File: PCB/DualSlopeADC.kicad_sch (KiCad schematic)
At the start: 25 parts, among them J2 Conn_01x02_Pin, J3 Conn_01x02_Pin, J5 Conn_01x02_Pin, J6 Conn_01x02_Pin, J7 Conn_01x02_Pin, J8 Conn_01x02_Pin, J9 Conn_01x02_Pin, U1 CH32V003FxPx, U2 ADR4533, U3 AD8605ARTZ-R2, U4 ADG419BRM, U5 LTC6752xSC6-4, U6 CA56-12EWA, U7 AD8656

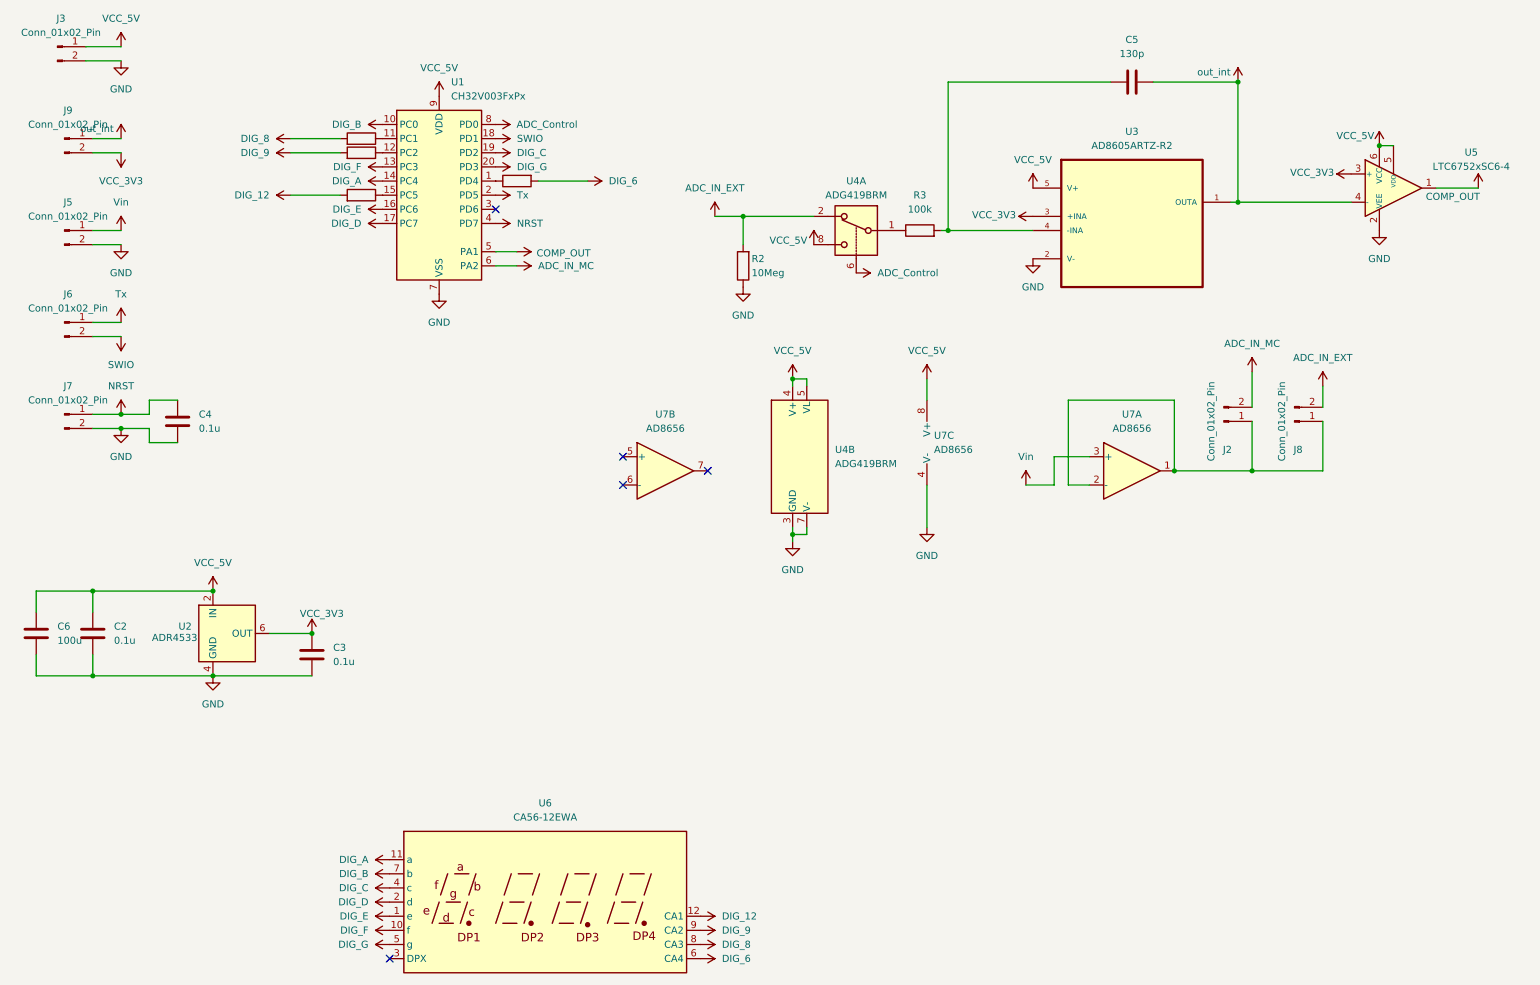
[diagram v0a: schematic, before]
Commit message: visulle sachen
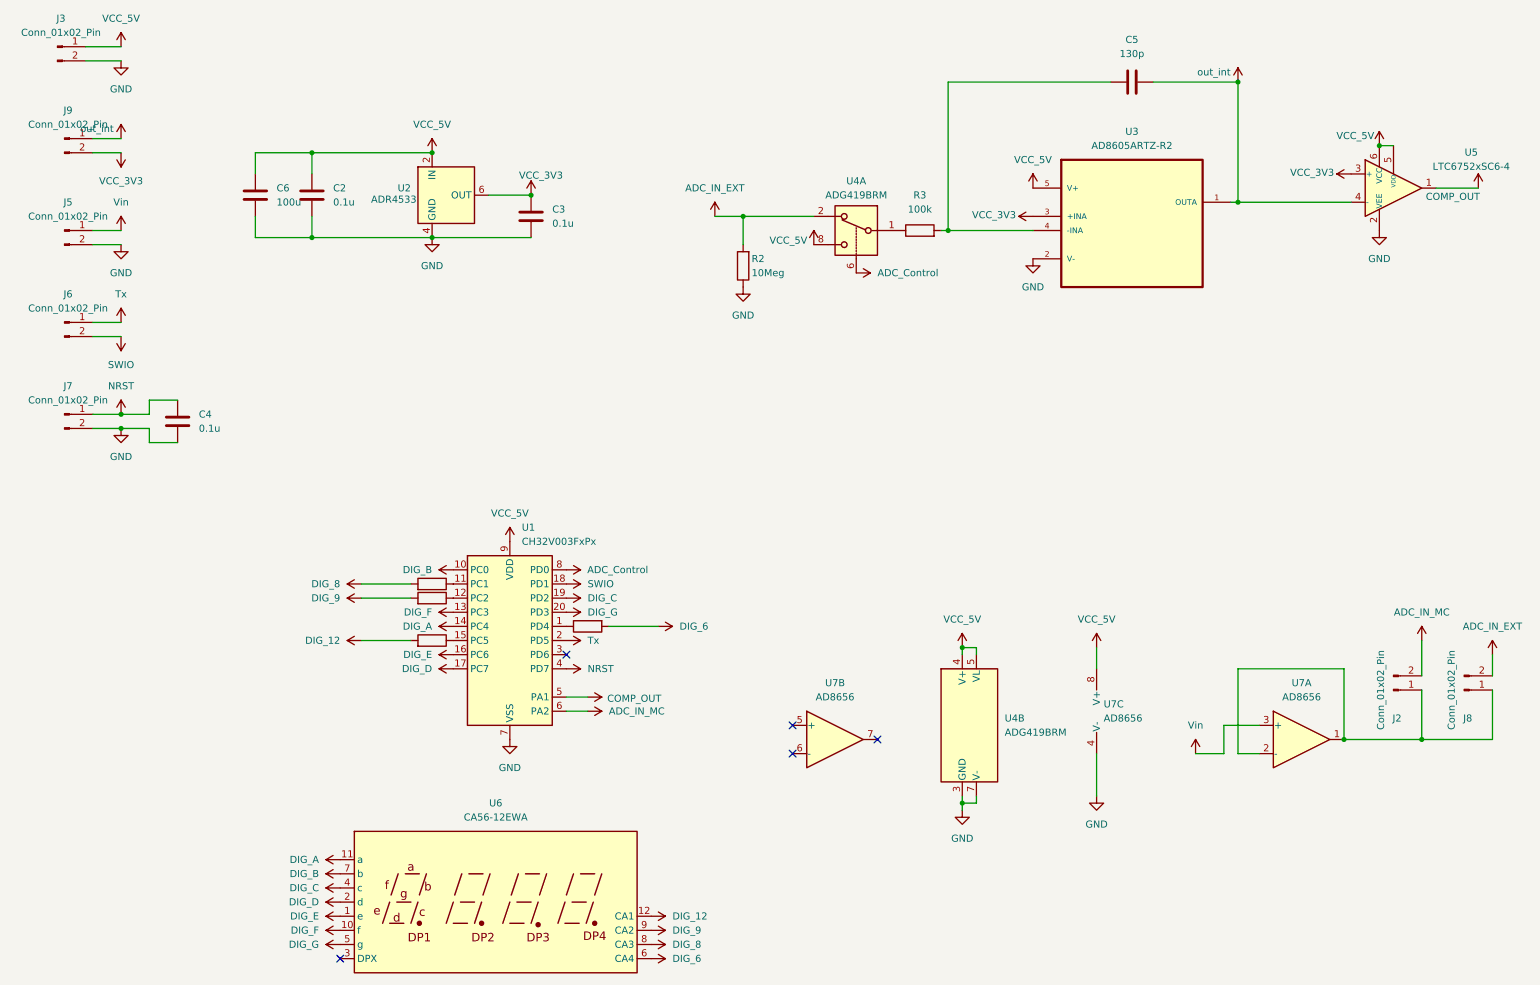
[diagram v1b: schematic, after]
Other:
- moved on the sheet: C2, C3, C6, J2, J8, U1, U2, U4B, U6, U7A, U7B, U7C
